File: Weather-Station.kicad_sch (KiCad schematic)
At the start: 9 parts, among them J1 Conn_01x22, J2 Conn_01x22, J3 CN2, J4 CN3, J5 Conn_02x22_Odd_Even, J6 Conn_01x22, J7 Conn_01x06, U1 ESP32-S3-DevKitC, U2 X-NUCLEO-GFX01M2

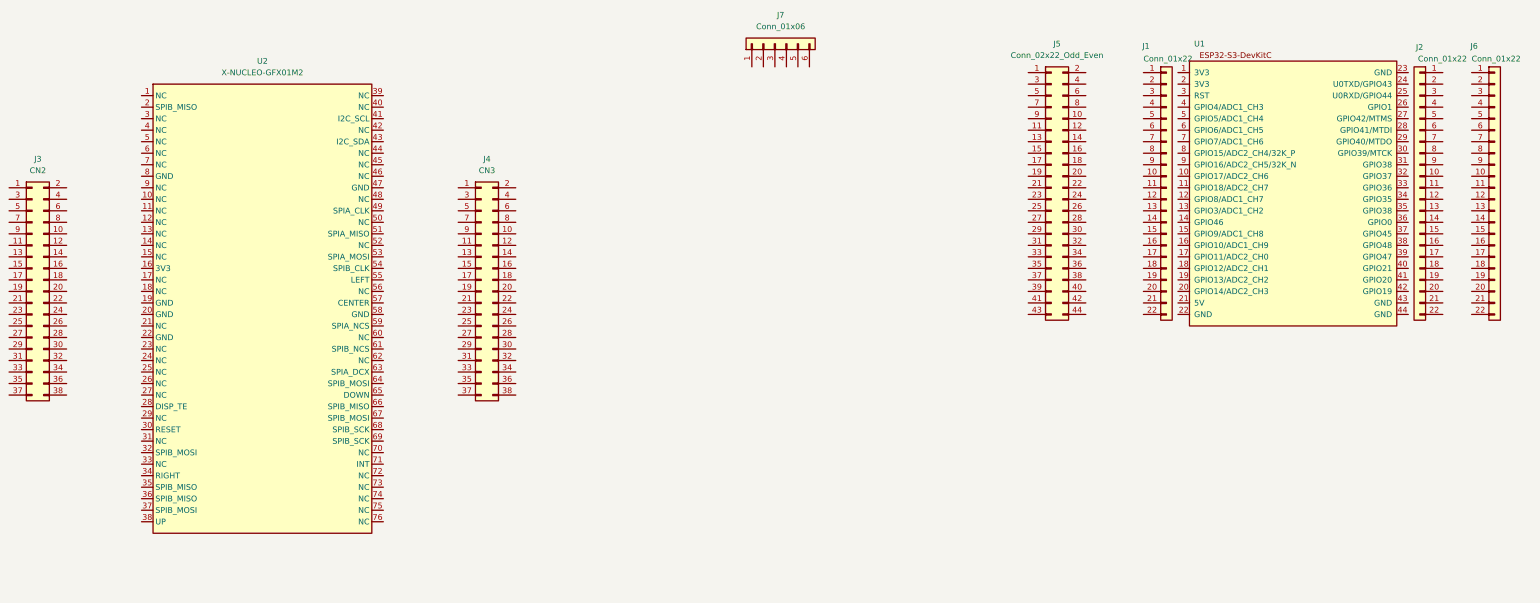
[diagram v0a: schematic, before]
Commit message: WIP: Started routing
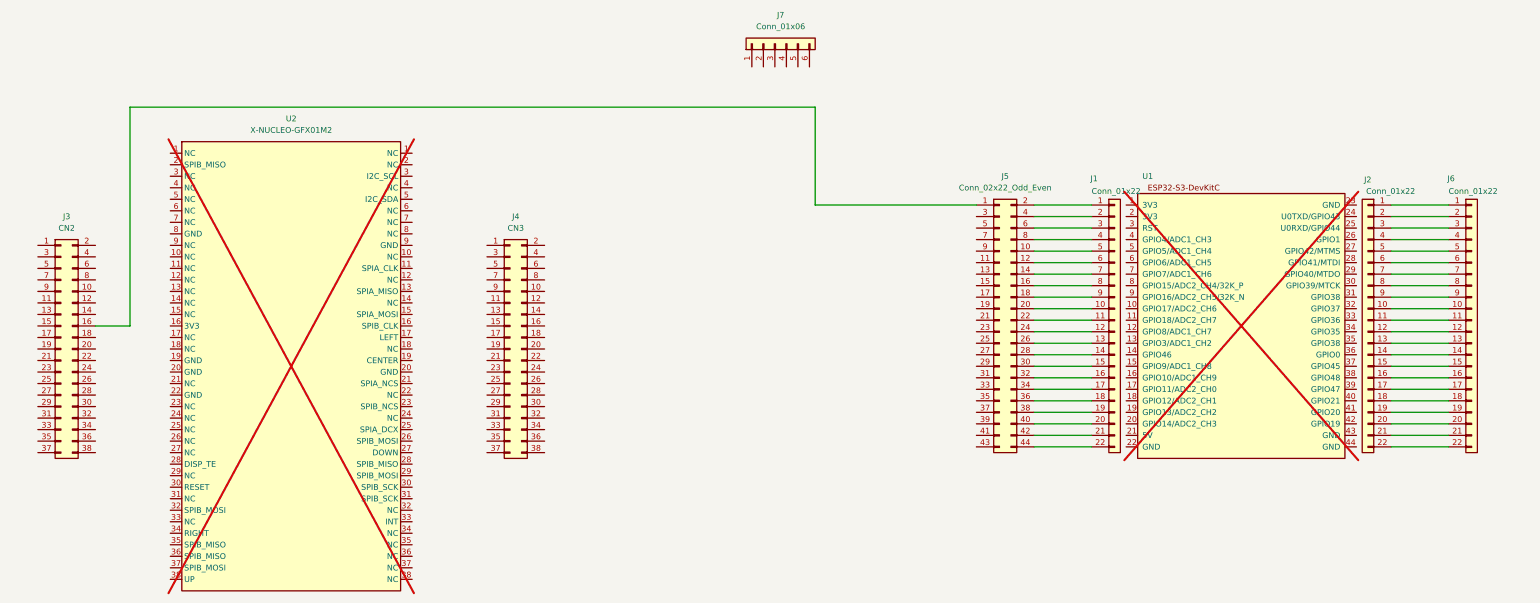
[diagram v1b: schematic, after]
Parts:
- U1, U2: now not fitted
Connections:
- net at J6.1 (Pin_1): now also J2.1 (Pin_1)
- net at J6.10 (Pin_10): now also J2.10 (Pin_10)
- net at J6.11 (Pin_11): now also J2.11 (Pin_11)
- net at J6.12 (Pin_12): now also J2.12 (Pin_12)
- net at J6.13 (Pin_13): now also J2.13 (Pin_13)
- net at J6.14 (Pin_14): now also J2.14 (Pin_14)
- net at J6.15 (Pin_15): now also J2.15 (Pin_15)
- net at J6.16 (Pin_16): now also J2.16 (Pin_16)
- net at J6.17 (Pin_17): now also J2.17 (Pin_17)
- net at J6.18 (Pin_18): now also J2.18 (Pin_18)
- net at J6.19 (Pin_19): now also J2.19 (Pin_19)
- net at J6.2 (Pin_2): now also J2.2 (Pin_2)
- net at J6.20 (Pin_20): now also J2.20 (Pin_20)
- net at J6.21 (Pin_21): now also J2.21 (Pin_21)
- net at J6.22 (Pin_22): now also J2.22 (Pin_22)
- net at J6.3 (Pin_3): now also J2.3 (Pin_3)
- net at J6.4 (Pin_4): now also J2.4 (Pin_4)
- net at J6.5 (Pin_5): now also J2.5 (Pin_5)
- net at J6.6 (Pin_6): now also J2.6 (Pin_6)
- net at J6.7 (Pin_7): now also J2.7 (Pin_7)
- net at J6.8 (Pin_8): now also J2.8 (Pin_8)
- net at J6.9 (Pin_9): now also J2.9 (Pin_9)
- net at J5.1 (Pin_1): now also J3.16 (Pin_16)
- net at J5.10 (Pin_10): now also J1.5 (Pin_5)
- net at J5.12 (Pin_12): now also J1.6 (Pin_6)
- net at J5.14 (Pin_14): now also J1.7 (Pin_7)
- net at J5.16 (Pin_16): now also J1.8 (Pin_8)
- net at J5.18 (Pin_18): now also J1.9 (Pin_9)
- net at J5.2 (Pin_2): now also J1.1 (Pin_1)
- net at J5.20 (Pin_20): now also J1.10 (Pin_10)
- net at J5.22 (Pin_22): now also J1.11 (Pin_11)
- net at J5.24 (Pin_24): now also J1.12 (Pin_12)
- net at J5.26 (Pin_26): now also J1.13 (Pin_13)
- net at J5.28 (Pin_28): now also J1.14 (Pin_14)
- net at J5.30 (Pin_30): now also J1.15 (Pin_15)
- net at J5.32 (Pin_32): now also J1.16 (Pin_16)
- net at J5.34 (Pin_34): now also J1.17 (Pin_17)
- net at J5.36 (Pin_36): now also J1.18 (Pin_18)
- net at J5.38 (Pin_38): now also J1.19 (Pin_19)
- net at J5.4 (Pin_4): now also J1.2 (Pin_2)
- net at J5.40 (Pin_40): now also J1.20 (Pin_20)
- net at J5.42 (Pin_42): now also J1.21 (Pin_21)
- net at J5.44 (Pin_44): now also J1.22 (Pin_22)
- net at J5.6 (Pin_6): now also J1.3 (Pin_3)
- net at J5.8 (Pin_8): now also J1.4 (Pin_4)
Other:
- title: (none) -> Weather Station PCB
- moved on the sheet: J1, J2, J3, J4, J5, J6
